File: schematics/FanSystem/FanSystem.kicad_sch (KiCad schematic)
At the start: 4 parts, among them M1 Fan_CPU_4pin, U1 ESP32S WROOM, U2 Oiyagai Breadboard Power Modu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, U3 AXLHNITI 60W 12V Inverter

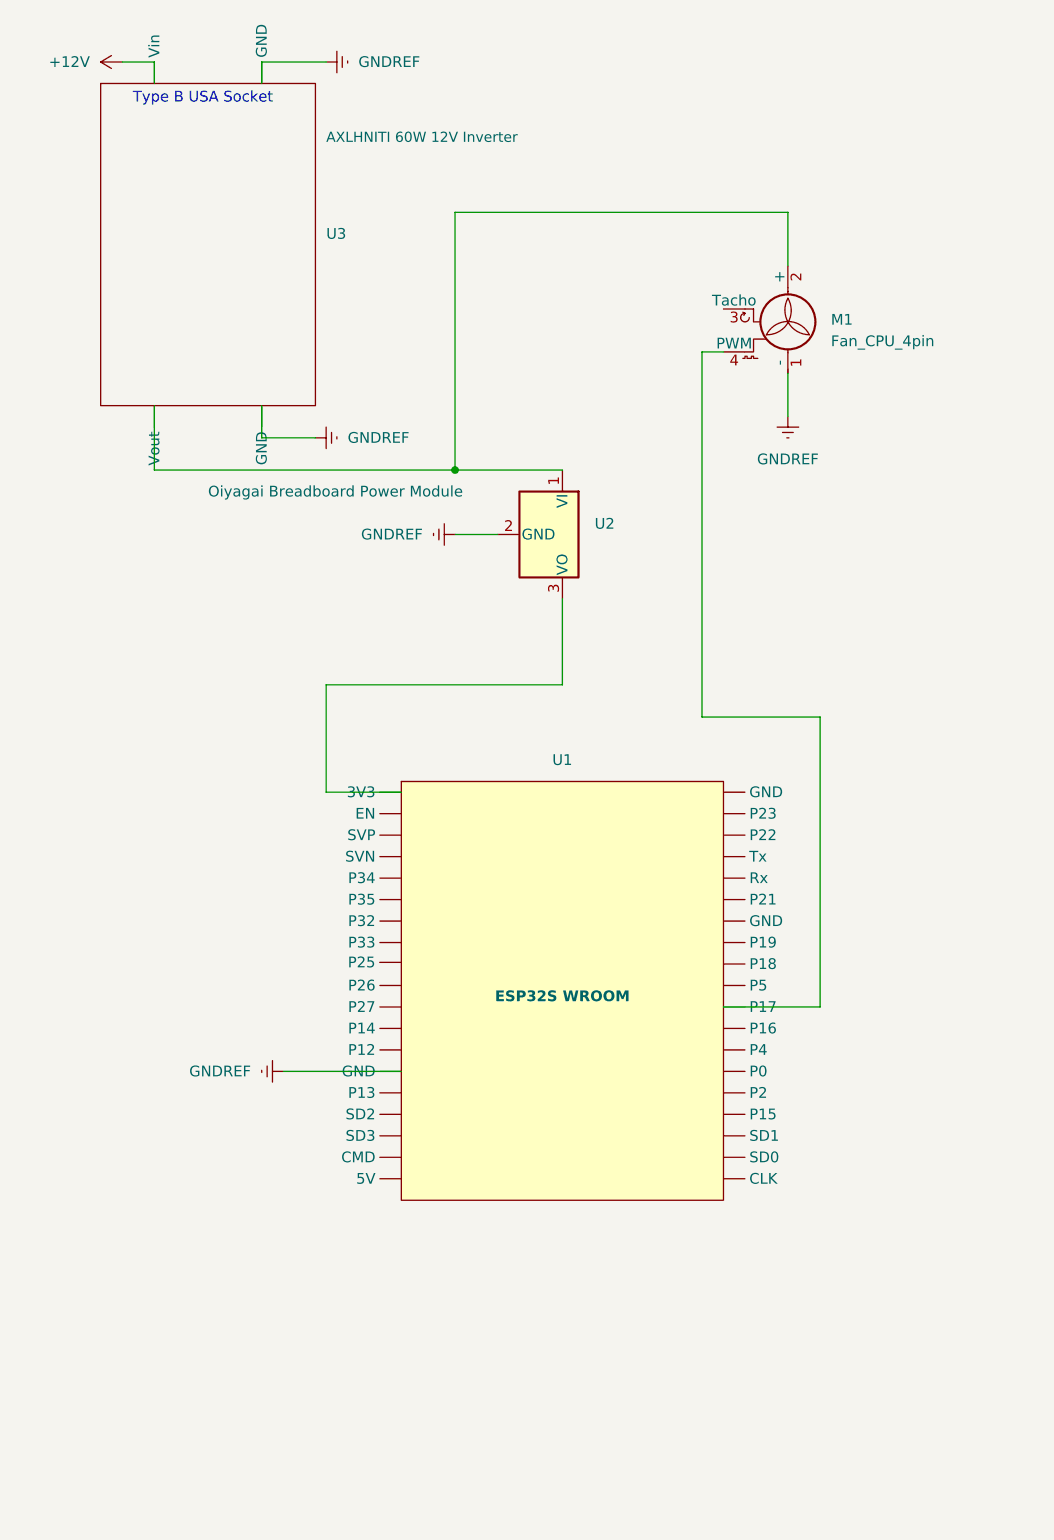
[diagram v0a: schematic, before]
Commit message: Updated Schematic Drawings
Schematics have been updated to the current build status of the project.
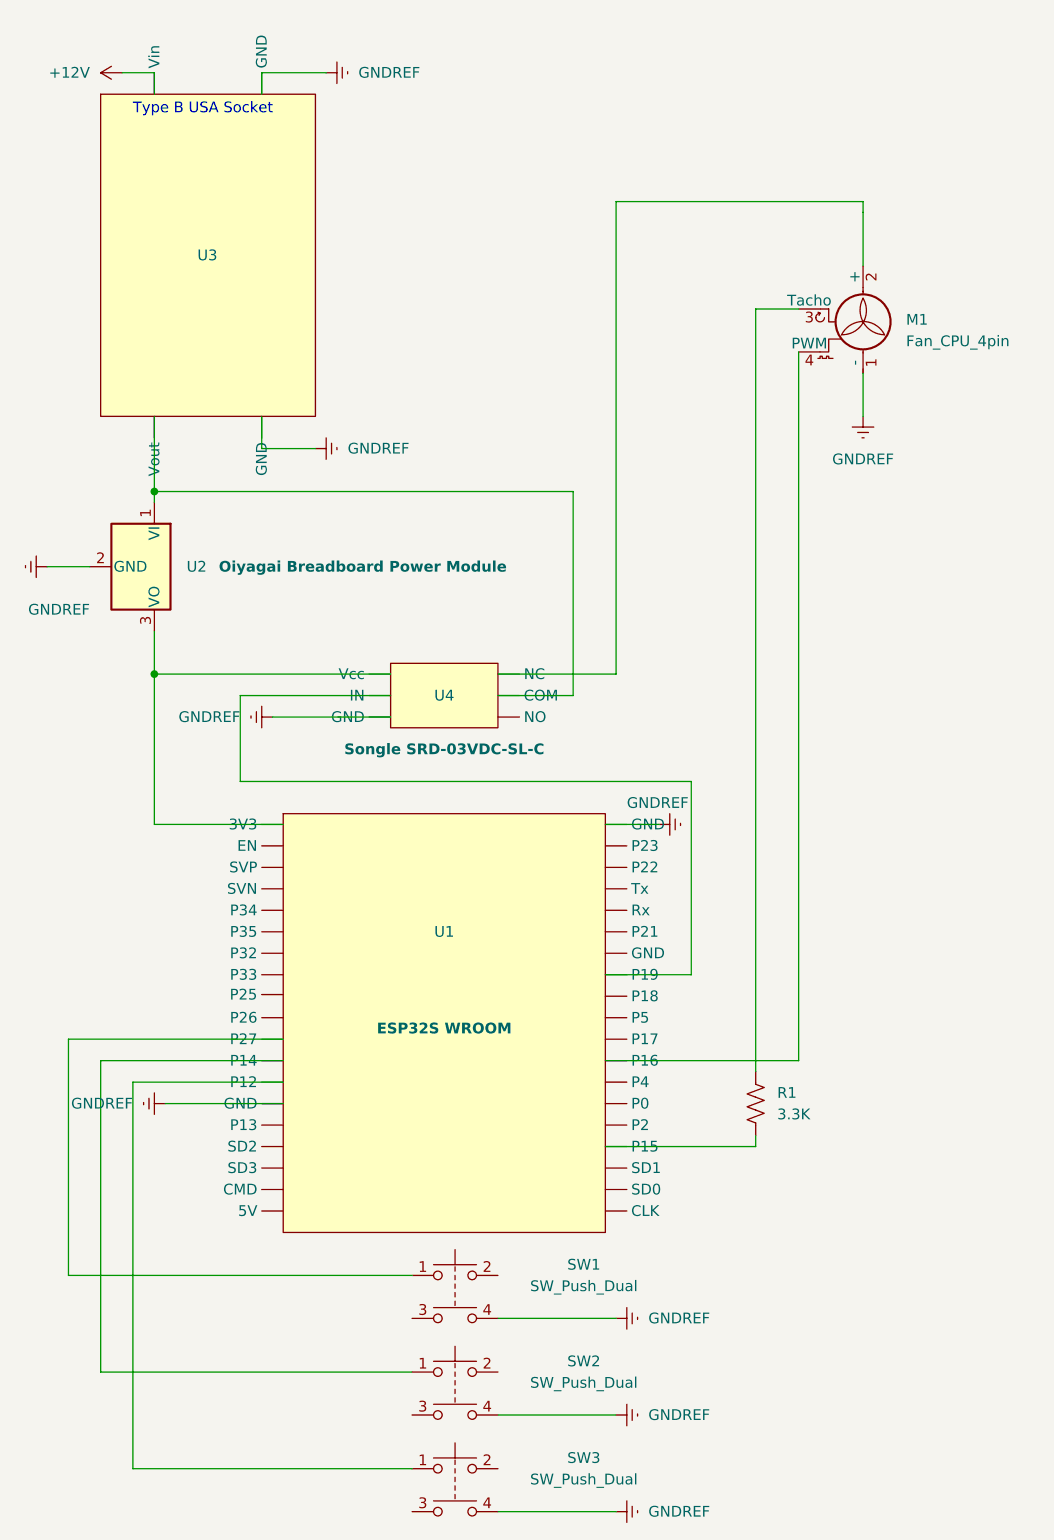
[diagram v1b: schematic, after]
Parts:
- added R1: 3.3K, symbol Device:R_US
- added SW1, SW2, SW3: SW_Push_Dual, symbol Switch:SW_Push_Dual
- added U4: Songle SRD-03VDC-SL-C, symbol 1A-Power:Songle
- U3: value AXLHNITI 60W 12V Inverter -> ~
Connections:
- net GNDREF: now also SW1.4, SW2.4, SW3.4, U4. (Vcc)
- net at U1. (Tx), U2.3 (VO): now also U4. (Vcc)
- net at M1.3 (Tacho): now also R1.1
- new net: SW3.1, U1. (Tx)
- new net: SW2.1, U1. (Tx)
- new net: U1. (Tx), U4. (Vcc)
- new net: R1.2, U1. (Tx)
- new net: SW1.1, U1. (Tx)
- new net: U2.1 (VI), U3. (Vout), U4. (Vcc)
- new net: M1.2 (+), U4. (Vcc)
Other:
- title: (none) -> Fan Control Device
- moved on the sheet: M1, U1, U2
